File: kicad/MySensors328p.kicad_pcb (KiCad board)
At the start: 2 copper layers, 27 x 18 mm, 22 parts, among them J1 U.FL, J2 U.FL, P1 HEADER_2x7, P2 HEADER_2x7, U1 NRF24L01, U3 ATmega328P-AU, Y1 16 MHz

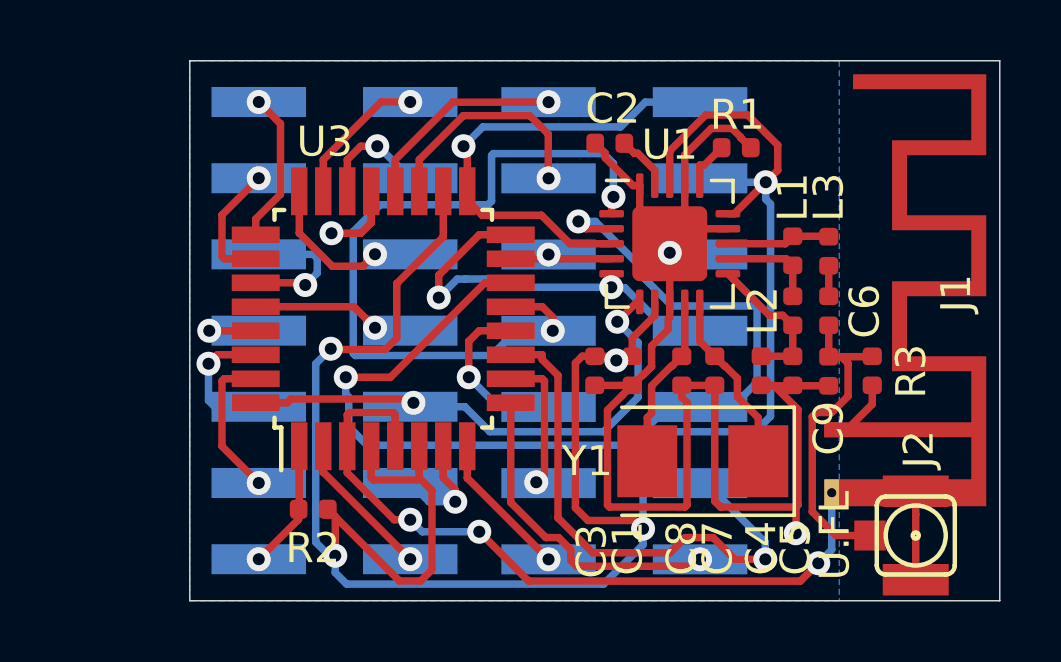
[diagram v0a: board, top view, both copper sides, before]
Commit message: Add files via upload
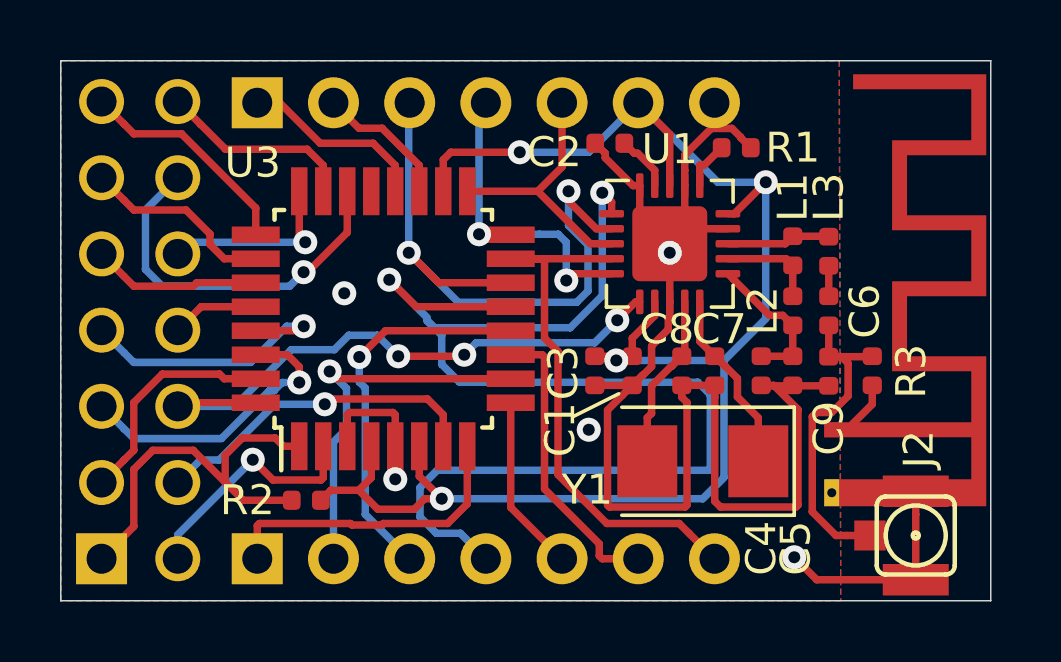
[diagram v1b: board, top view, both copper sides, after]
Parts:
- added P3: HEADER_1x7, Connector_PinHeader_2.54mm:PinHeader_1x07_P2.54mm_Vertical, B.Cu at (131.4, 92.5)
- P1: value HEADER_2x7 -> HEADER_1x7; footprint Connector_PinHeader_2.54mm:PinHeader_2x07_P2.54mm_Vertical_SMD -> Connector_PinHeader_2.54mm:PinHeader_1x07_P2.54mm_Vertical
- P2: footprint Connector_PinHeader_2.54mm:PinHeader_2x07_P2.54mm_Vertical_SMD -> Connector_PinHeader_2.54mm:PinHeader_2x07_P2.54mm_Vertical
- moved P1 14.4 mm to (131.4, 107.7), turned to 270 degrees
- moved P2 10.9 mm to (126.3, 107.7)
- moved R2 0.38 mm to (133.1, 105.8)
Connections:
- P1 pad 4: Net-(P1-Pad4) -> CE
- P1 pad 6: CSN -> Net-(P1-Pad6)
- P1 pad 7: CE -> MOSI
- U3 pad 10: Net-(P1-Pad3) -> Net-(P1-Pad2)
- U3 pad 11: Net-(P1-Pad4) -> Net-(P1-Pad6)
- U3 pad 12: Net-(P1-Pad5) -> Net-(P1-Pad3)
- U3 pad 19: Net-(P1-Pad11) -> Net-(P3-Pad2)
- U3 pad 20: Net-(P1-Pad13) -> Net-(P3-Pad1)
- U3 pad 9: Net-(P1-Pad2) -> Net-(P1-Pad5)
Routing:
- net 3,3V: track 79.0 -> 54.7 mm, vias 5 -> 4
- net GND: track 78.2 -> 59.4 mm, vias 6 -> 5
- net CE: track 25.4 -> 44.2 mm
- net Net-(P1-Pad4): track 18.3 -> 0.00 mm, vias 1 -> 0
- net MOSI: track 3.63 -> 18.2 mm, vias 1 -> 0
- net CSN: track 34.2 -> 21.4 mm
- net Net-(P1-Pad6): track 0.00 -> 9.88 mm
- net Net-(P2-Pad1): track 4.32 -> 13.4 mm, vias 1 -> 0
- net Net-(P1-Pad3): track 4.64 -> 12.8 mm
- net Net-(P2-Pad12): track 4.85 -> 12.6 mm
- net Net-(P1-Pad11): track 7.69 -> 0.00 mm, vias 1 -> 0
- net Net-(P2-Pad4): track 3.77 -> 11.3 mm
- net Net-(P1-Pad13): track 6.96 -> 0.00 mm, vias 1 -> 0
- net SCK: track 15.8 -> 8.82 mm, vias 1 -> 0
- net Net-(P3-Pad1): track 0.00 -> 6.33 mm
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- added copper zone on F.Cu, net GND
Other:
- board size 27 x 18 mm -> 31 x 18 mm
- board text added: "/PB1"
- board text added: "AREF"
- board text added: "CE"
- board text added: "IRQ"
- board text added: "MISO"
- board text added: "MOSI/PB3"
- board text added: "PB4/"
- board text added: "PD2"
- board text added: "PD3"
- board text added: "VDD"
- board text removed: "AERF"
- board text removed: "PB1 /CE"
- board text removed: "PB3/ MOSI"
- board text removed: "PB4/MISO"
- board text removed: "PD2/ IRQ"
- board text removed: "PD3/ RES"
- board text removed: "VCC"
